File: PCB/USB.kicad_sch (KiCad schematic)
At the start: 11 parts, among them J6 USB4510-03-1-A_REVA, U13 HSP051-4M10

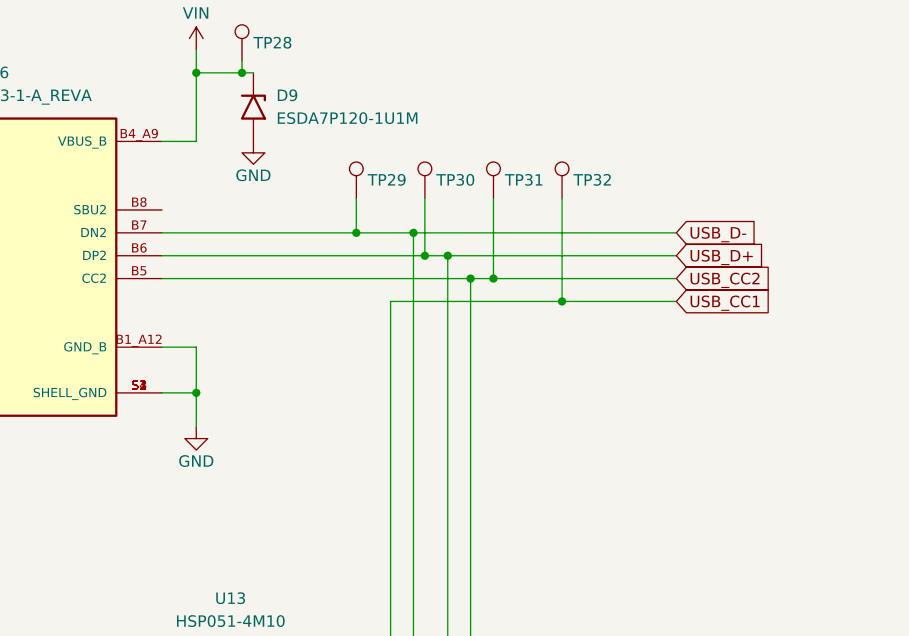
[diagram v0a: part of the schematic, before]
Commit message: update
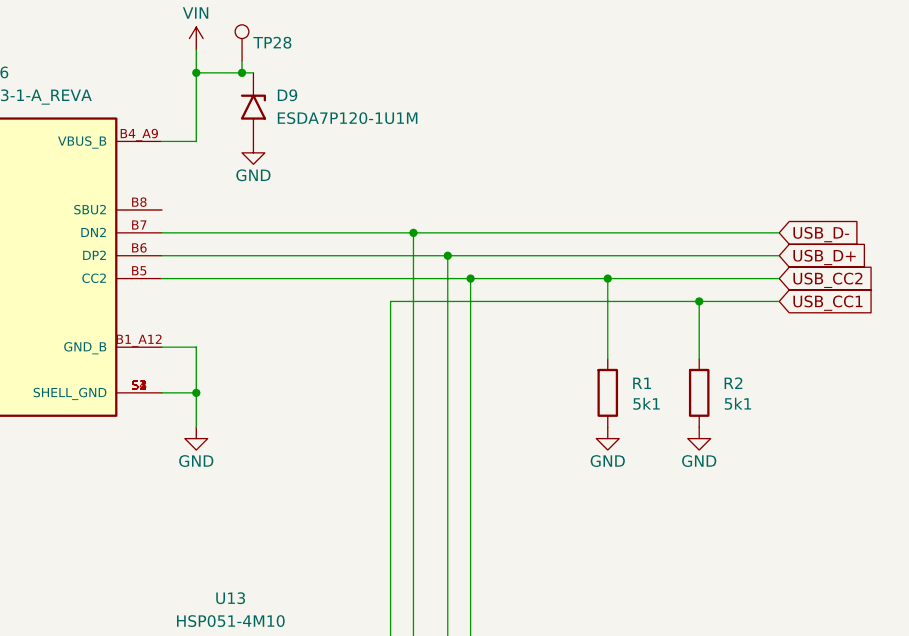
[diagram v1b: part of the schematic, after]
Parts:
- removed TP29, TP30, TP31, TP32: TestPoint, lib:TP_0.5, symbol Connector:TestPoint
- added R1, R2: 5k1, Resistor_SMD:R_0402_1005Metric, symbol Device:R
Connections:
- net GND: now also R1.1, R2.1
- net USB_CC1: now also R2.2
- net USB_CC2: now also R1.2
